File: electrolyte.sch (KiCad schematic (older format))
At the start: 41 parts

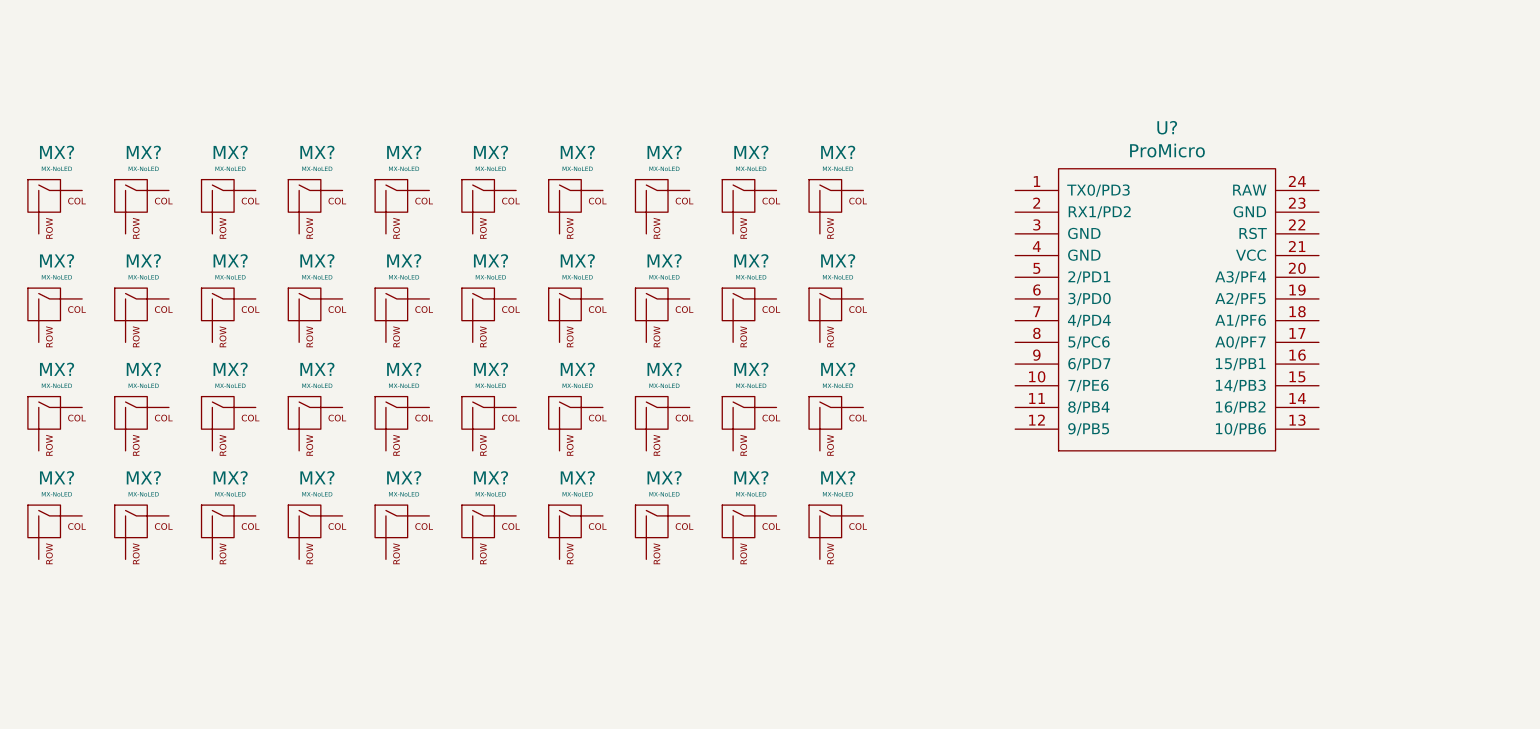
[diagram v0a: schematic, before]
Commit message: more work on the design
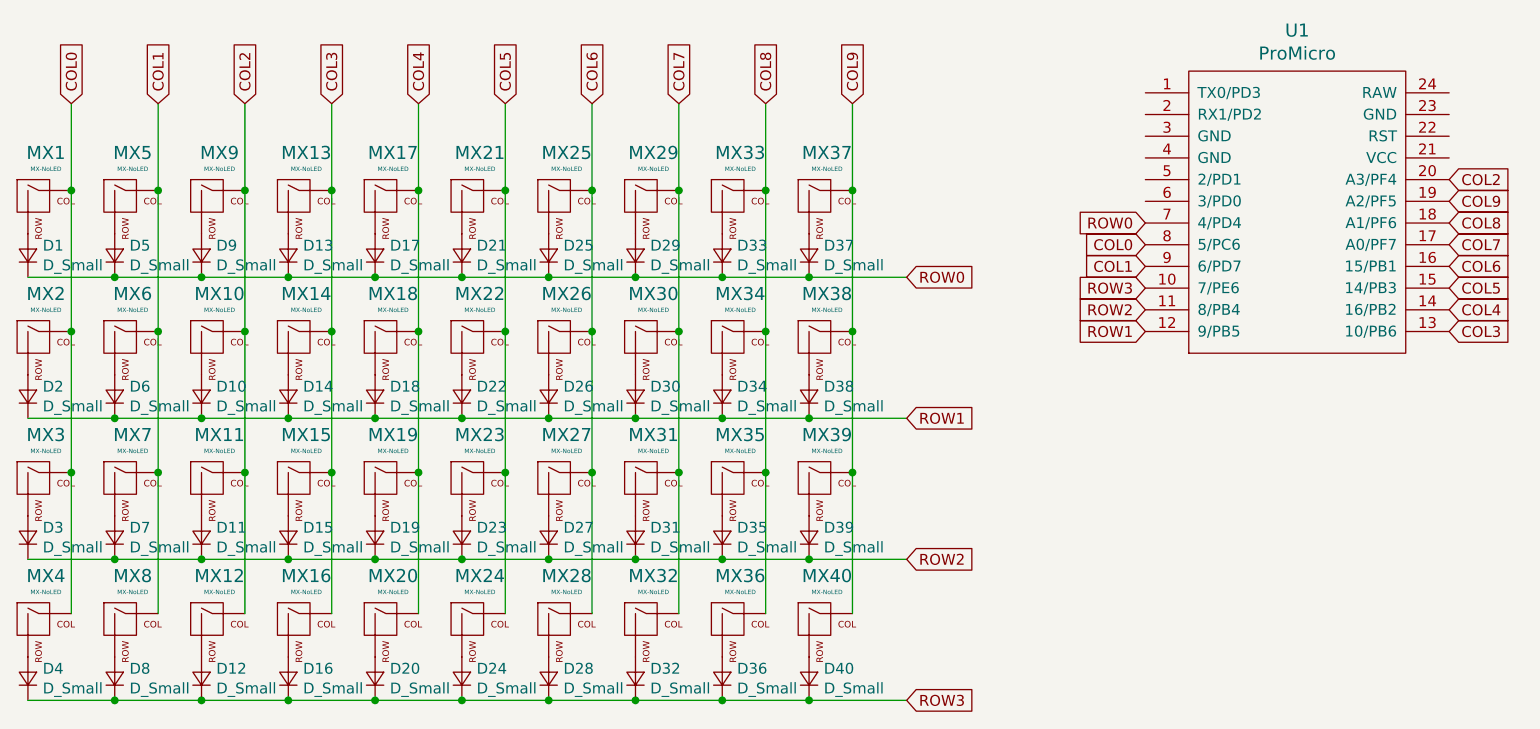
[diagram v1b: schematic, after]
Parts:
- added D1, D10, D11, D12, D13, D14, D15, D16, D17, D18, D19, D2, D20, D21, D22, D23, D24, D25, D26, D27, D28, D29, D3, D30, D31, D32, D33, D34, D35, D36, D37, D38, D39, D4, D40, D5, D6, D7, D8, D9: D_Small, Keebio-Parts:Diode-Hybrid-Back, symbol Device:D_Small
- MX1, MX10, MX11, MX12, MX13, MX14, MX15, MX16, MX17, MX18, MX19, MX2, MX20, MX21, MX22, MX23, MX24, MX25, MX26, MX27, MX28, MX29, MX3, MX30, MX31, MX32, MX33, MX34, MX35, MX36, MX37, MX38, MX39, MX4, MX40, MX5, MX6, MX7, MX8, MX9: renamed from MX?; footprint (none) -> MX_Only:MXOnly-1U-NoLED
- U1: renamed from U?; footprint (none) -> Keebio-Parts:ArduinoProMicro
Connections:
- net ROW3: now reaches U1.10 (7/PE6)
- net ROW3: now also D12.1 (K), D16.1 (K), D20.1 (K), D24.1 (K), D28.1 (K), D32.1 (K), D36.1 (K), D4.1 (K), D40.1 (K), D8.1 (K)
- net ROW2: now reaches U1.11 (8/PB4)
- net ROW2: now also D11.1 (K), D15.1 (K), D19.1 (K), D23.1 (K), D27.1 (K), D3.1 (K), D31.1 (K), D35.1 (K), D39.1 (K), D7.1 (K)
- net ROW1: now reaches U1.12 (9/PB5)
- net ROW1: now also D10.1 (K), D14.1 (K), D18.1 (K), D2.1 (K), D22.1 (K), D26.1 (K), D30.1 (K), D34.1 (K), D38.1 (K), D6.1 (K)
- net COL3: now reaches U1.13 (10/PB6)
- net COL3: now also MX13.1 (COL), MX14.1 (COL), MX15.1 (COL), MX16.1 (COL)
- net COL4: now reaches U1.14 (16/PB2)
- net COL4: now also MX17.1 (COL), MX18.1 (COL), MX19.1 (COL), MX20.1 (COL)
- net COL5: now reaches U1.15 (14/PB3)
- net COL5: now also MX21.1 (COL), MX22.1 (COL), MX23.1 (COL), MX24.1 (COL)
- net COL6: now reaches U1.16 (15/PB1)
- net COL6: now also MX25.1 (COL), MX26.1 (COL), MX27.1 (COL), MX28.1 (COL)
- net COL7: now reaches U1.17 (A0/PF7)
- net COL7: now also MX29.1 (COL), MX30.1 (COL), MX31.1 (COL), MX32.1 (COL)
- net COL8: now reaches U1.18 (A1/PF6)
- net COL8: now also MX33.1 (COL), MX34.1 (COL), MX35.1 (COL), MX36.1 (COL)
- net COL9: now reaches U1.19 (A2/PF5)
- net COL9: now also MX37.1 (COL), MX38.1 (COL), MX39.1 (COL), MX40.1 (COL)
- net COL2: now reaches U1.20 (A3/PF4)
- net COL2: now also MX10.1 (COL), MX11.1 (COL), MX12.1 (COL), MX9.1 (COL)
- net ROW0: now reaches U1.7 (4/PD4)
- net ROW0: now also D1.1 (K), D13.1 (K), D17.1 (K), D21.1 (K), D25.1 (K), D29.1 (K), D33.1 (K), D37.1 (K), D5.1 (K), D9.1 (K)
- net COL0: now reaches U1.8 (5/PC6)
- net COL0: now also MX1.1 (COL), MX2.1 (COL), MX3.1 (COL), MX4.1 (COL)
- net COL1: now reaches U1.9 (6/PD7)
- net COL1: now also MX5.1 (COL), MX6.1 (COL), MX7.1 (COL), MX8.1 (COL)
- net at MX1.2 (ROW): now also D1.2 (A)
- net at MX2.2 (ROW): now also D2.2 (A)
- net at MX3.2 (ROW): now also D3.2 (A)
- net at MX4.2 (ROW): now also D4.2 (A)
- net at MX5.2 (ROW): now also D5.2 (A)
- net at MX6.2 (ROW): now also D6.2 (A)
- net at MX7.2 (ROW): now also D7.2 (A)
- net at MX8.2 (ROW): now also D8.2 (A)
- net at MX9.2 (ROW): now also D9.2 (A)
- net at MX10.2 (ROW): now also D10.2 (A)
- net at MX11.2 (ROW): now also D11.2 (A)
- net at MX12.2 (ROW): now also D12.2 (A)
- net at MX13.2 (ROW): now also D13.2 (A)
- net at MX14.2 (ROW): now also D14.2 (A)
- net at MX15.2 (ROW): now also D15.2 (A)
- net at MX16.2 (ROW): now also D16.2 (A)
- net at MX17.2 (ROW): now also D17.2 (A)
- net at MX18.2 (ROW): now also D18.2 (A)
- net at MX19.2 (ROW): now also D19.2 (A)
- net at MX20.2 (ROW): now also D20.2 (A)
- net at MX21.2 (ROW): now also D21.2 (A)
- net at MX22.2 (ROW): now also D22.2 (A)
- net at MX23.2 (ROW): now also D23.2 (A)
- net at MX24.2 (ROW): now also D24.2 (A)
- net at MX25.2 (ROW): now also D25.2 (A)
- net at MX26.2 (ROW): now also D26.2 (A)
- net at MX27.2 (ROW): now also D27.2 (A)
- net at MX28.2 (ROW): now also D28.2 (A)
- net at MX29.2 (ROW): now also D29.2 (A)
- net at MX30.2 (ROW): now also D30.2 (A)
- net at MX31.2 (ROW): now also D31.2 (A)
- net at MX32.2 (ROW): now also D32.2 (A)
- net at MX33.2 (ROW): now also D33.2 (A)
- net at MX34.2 (ROW): now also D34.2 (A)
- net at MX35.2 (ROW): now also D35.2 (A)
- net at MX36.2 (ROW): now also D36.2 (A)
- net at MX37.2 (ROW): now also D37.2 (A)
- net at MX38.2 (ROW): now also D38.2 (A)
- net at MX39.2 (ROW): now also D39.2 (A)
- net at MX40.2 (ROW): now also D40.2 (A)
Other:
- moved on the sheet: MX1, MX10, MX11, MX12, MX13, MX14, MX15, MX16, MX17, MX18, MX19, MX2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
